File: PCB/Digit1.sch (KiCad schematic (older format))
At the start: 1 part

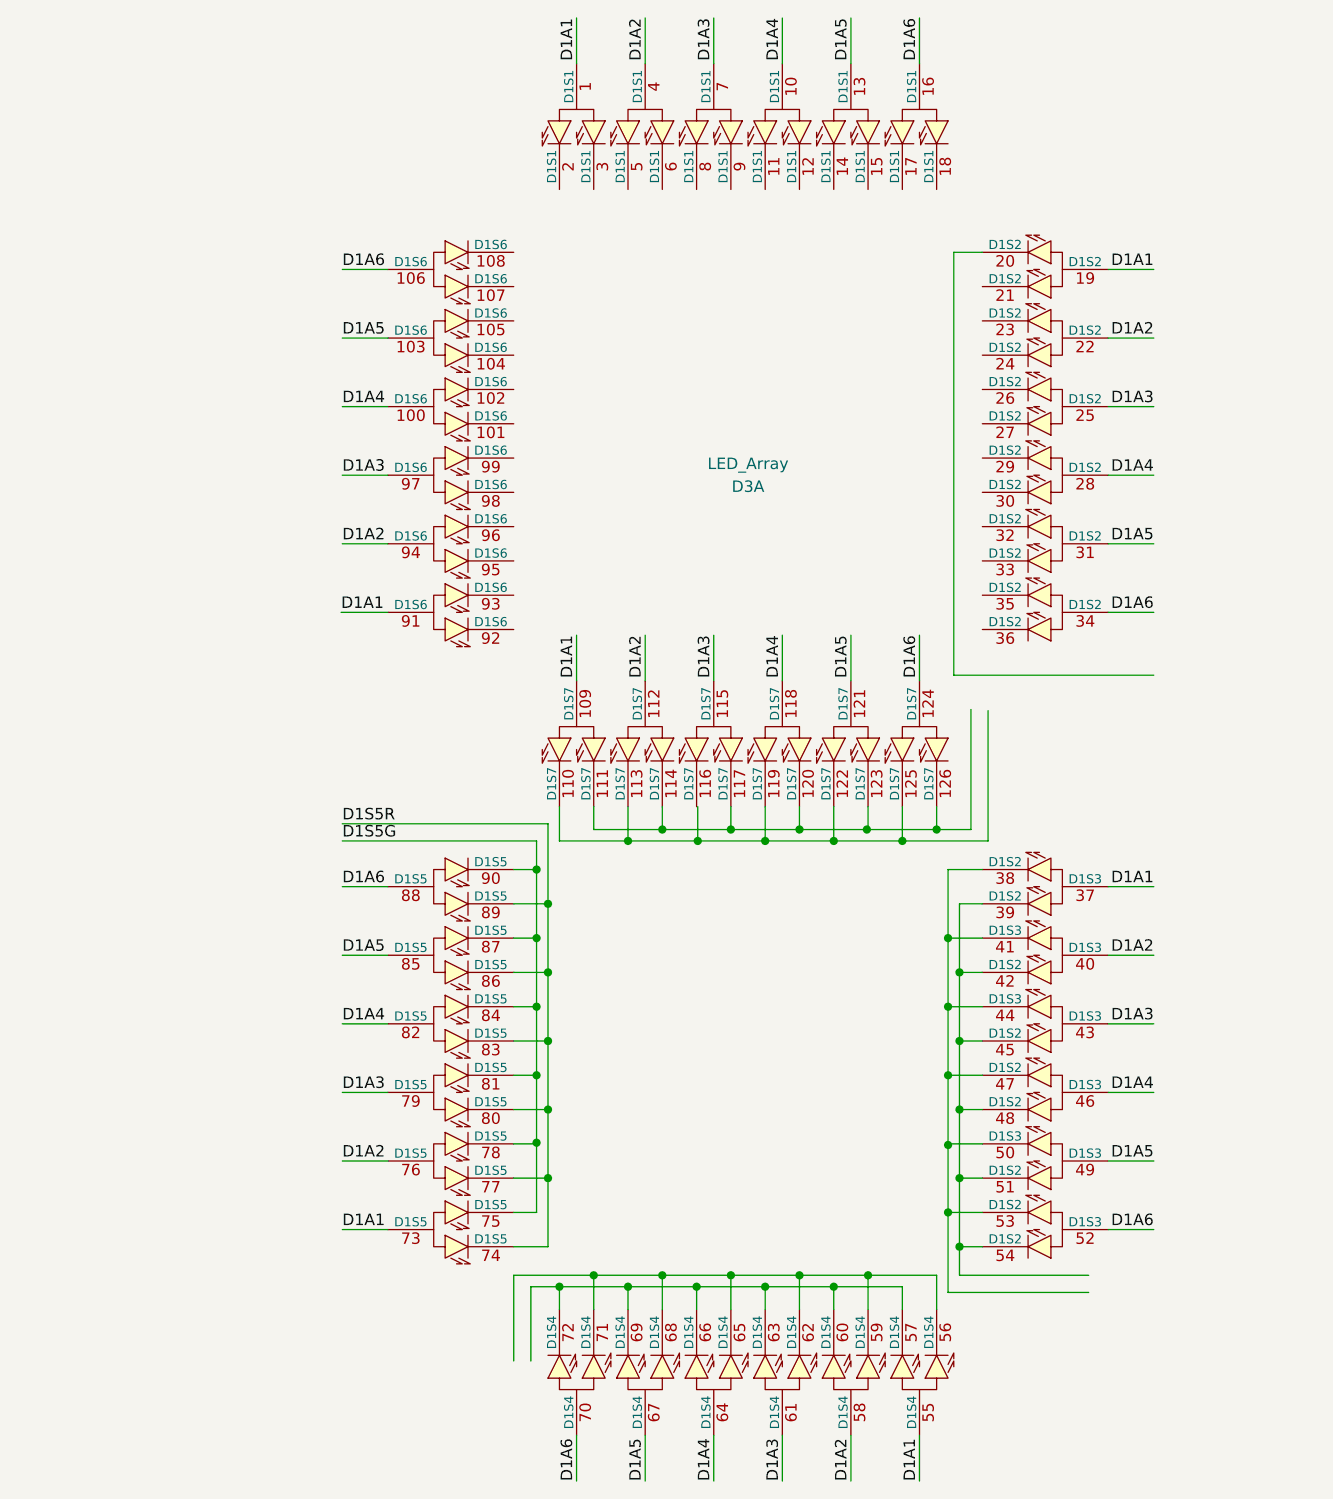
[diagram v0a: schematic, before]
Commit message: Worked on PCB
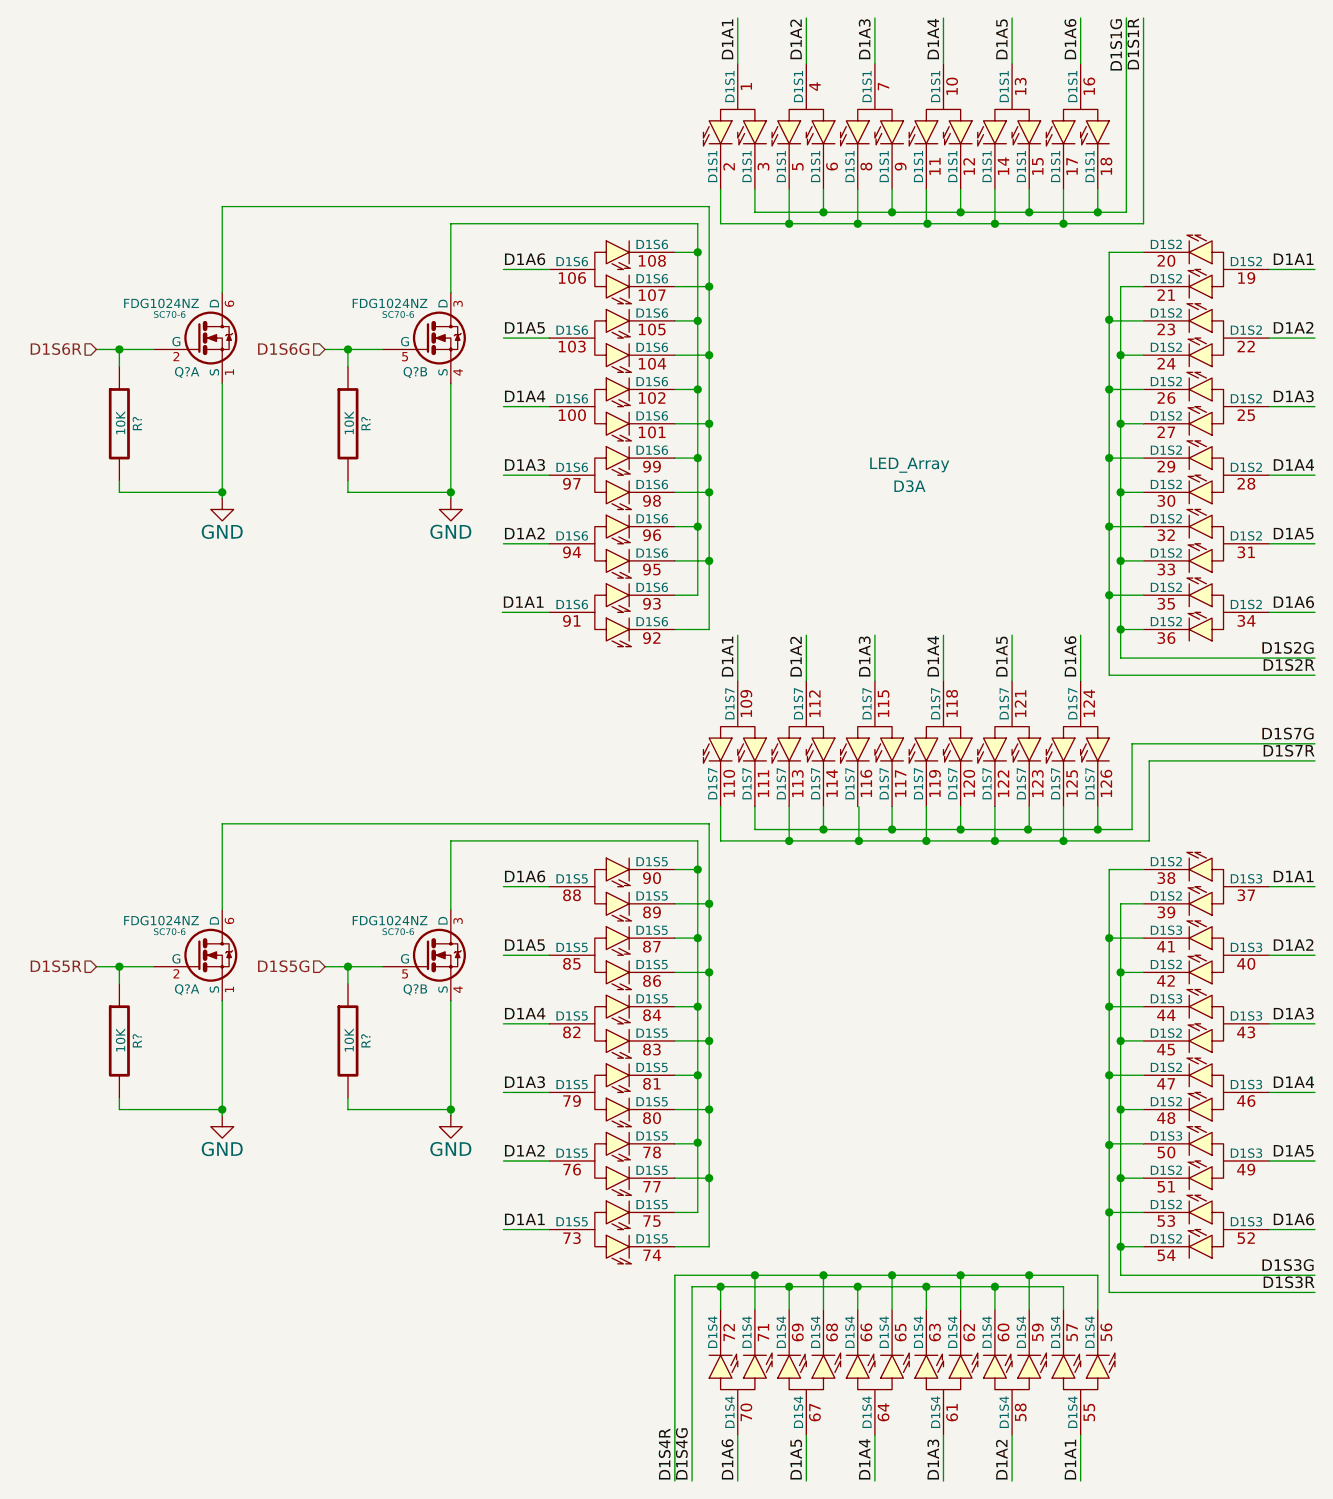
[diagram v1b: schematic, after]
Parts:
- added Q? (x4): FDG1024NZ, SC70-6, symbol FDG1024NZ
- added R? (x4): 10K, symbol R
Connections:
- net labels added: D1S1G, D1S1R, D1S2G, D1S2R, D1S3G, D1S3R, D1S4G, D1S4R, D1S6G, D1S6R, D1S7G, D1S7R, GND
- wire segments 152 -> 263
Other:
- moved on the sheet: D3A
